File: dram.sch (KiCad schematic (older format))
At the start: 23 parts

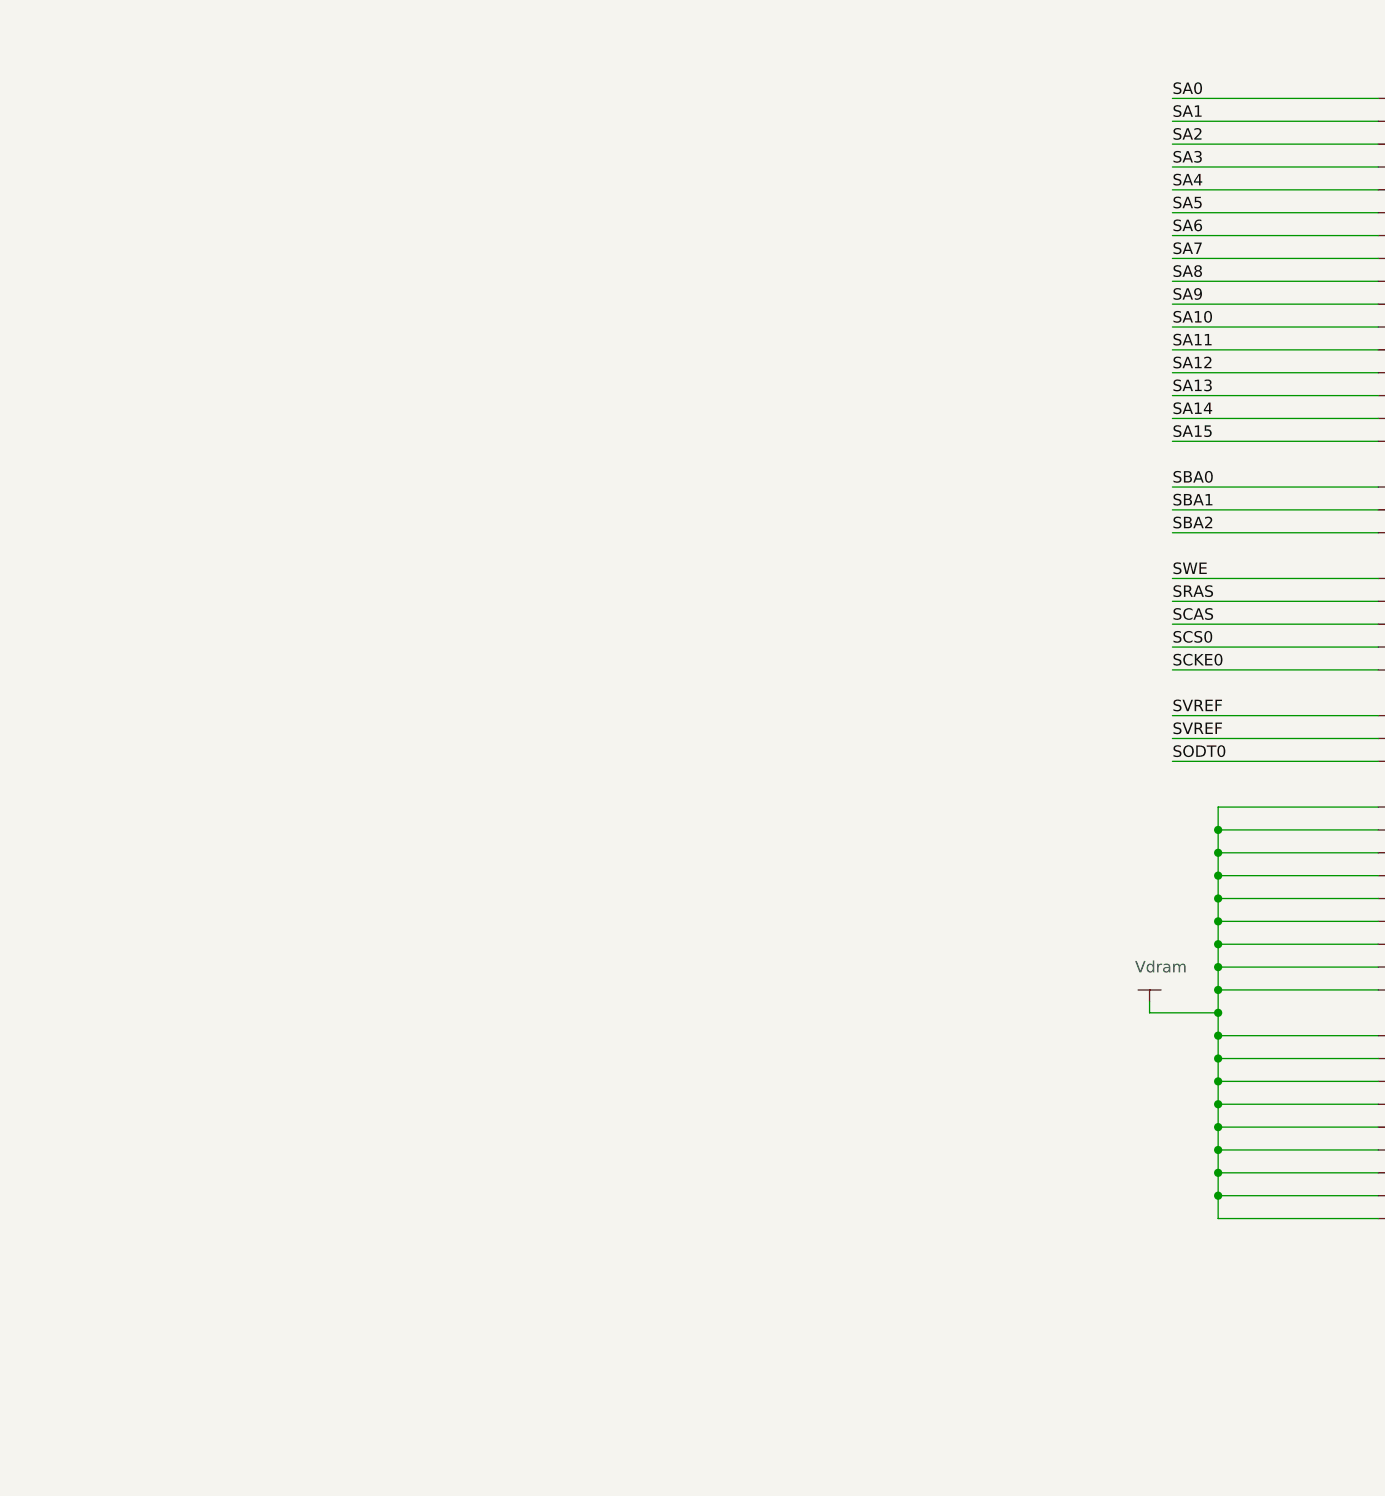
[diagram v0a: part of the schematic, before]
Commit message: update port sys,
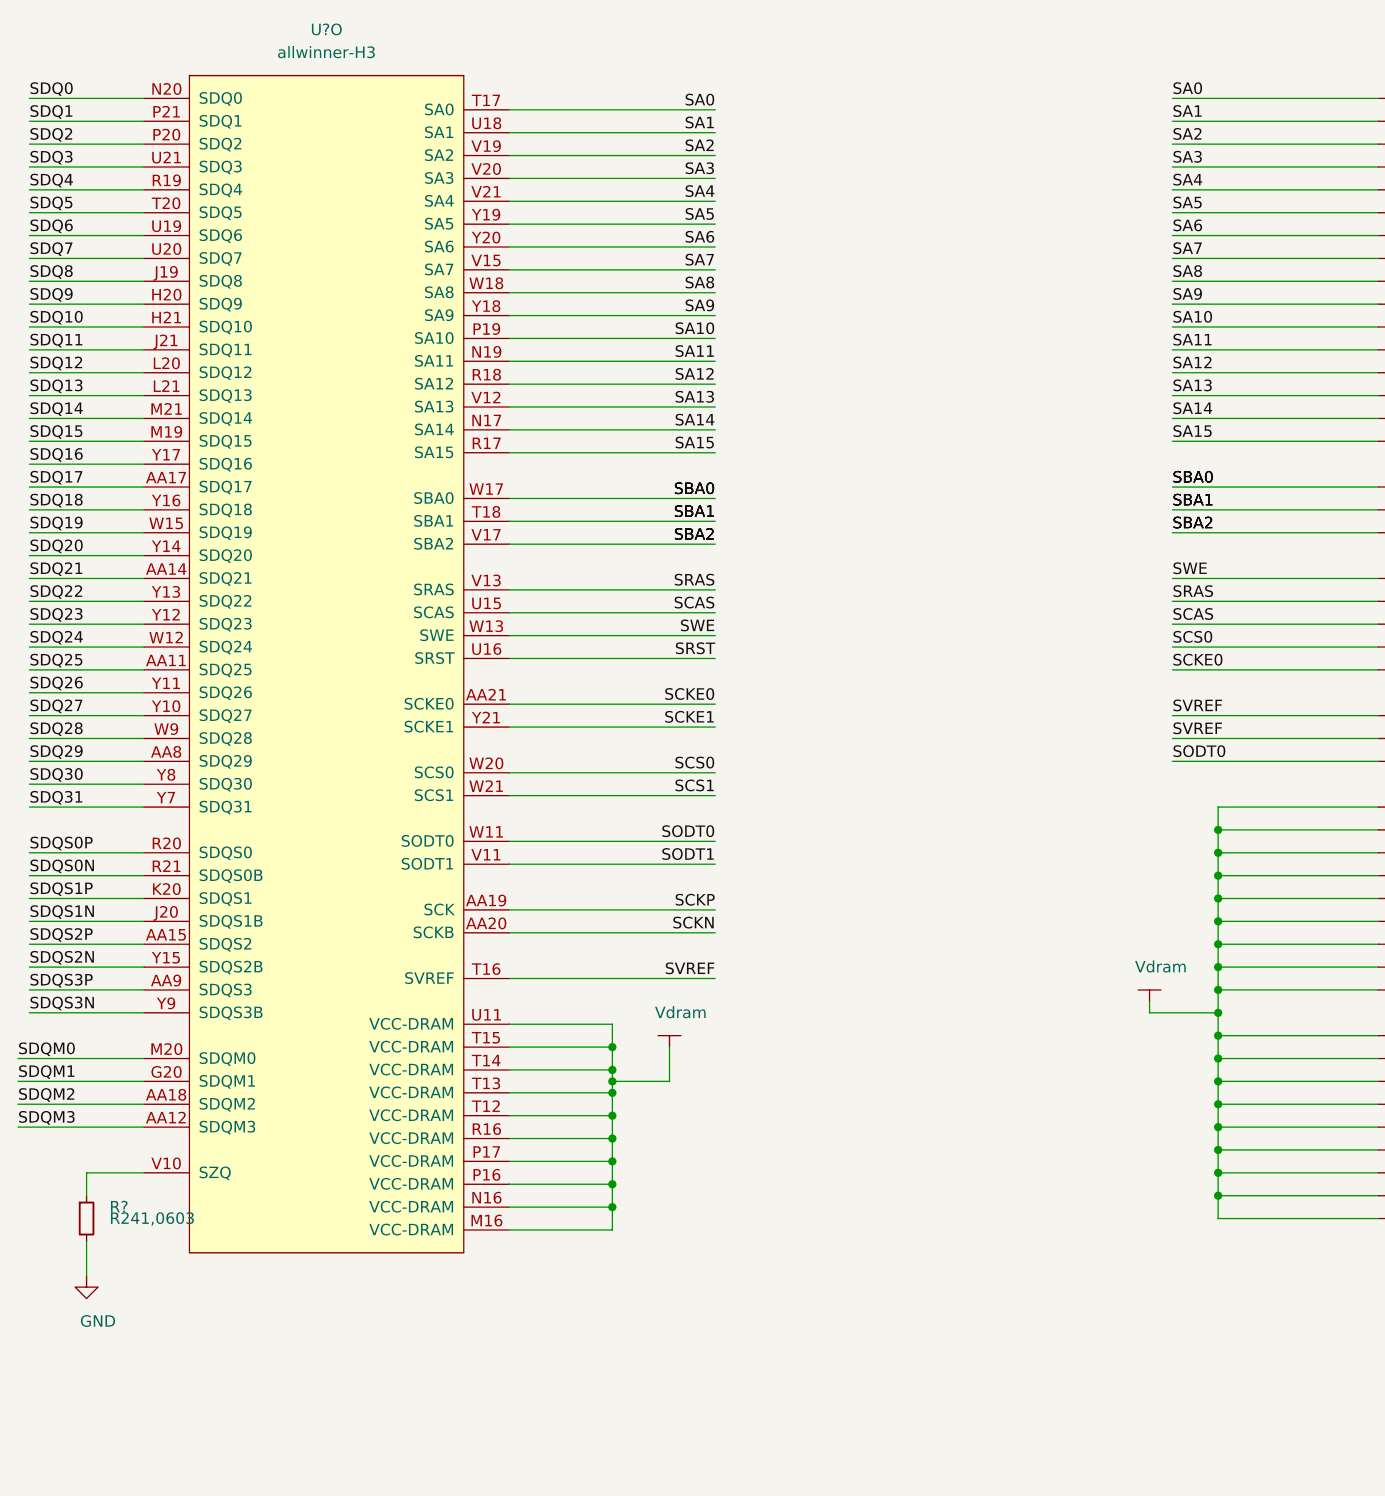
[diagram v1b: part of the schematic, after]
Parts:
- added R?: R241,0603, Resistor_SMD:R_0603_1608Metric_Pad1.05x0.95mm_HandSolder, symbol taobao-r:R241,0603
- added U?: allwinner-H3, symbol taobao-components:allwinner-H3
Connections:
- net GND: now also R?.2
- net SA0: now also U?.T17 (SA0)
- net SA1: now also U?.U18 (SA1)
- net SA10: now also U?.P19 (SA10)
- net SA11: now also U?.N19 (SA11)
- net SA12: now also U?.R18 (SA12)
- net SA13: now also U?.V12 (SA13)
- net SA14: now also U?.N17 (SA14)
- net SA15: now also U?.R17 (SA15)
- net SA2: now also U?.V19 (SA2)
- net SA3: now also U?.V20 (SA3)
- net SA4: now also U?.V21 (SA4)
- net SA5: now also U?.Y19 (SA5)
- net SA6: now also U?.Y20 (SA6)
- net SA7: now also U?.V15 (SA7)
- net SA8: now also U?.W18 (SA8)
- net SA9: now also U?.Y18 (SA9)
- net SBA0: now also U?.W17 (SBA0)
- net SBA1: now also U?.T18 (SBA1)
- net SBA2: now also U?.V17 (SBA2)
- net SCAS: now also U?.U15 (SCAS)
- net SCKE0: now also U?.AA21 (SCKE0)
- net SCKE1: now also U?.Y21 (SCKE1)
- net SCKN: now also U?.AA20 (SCKB)
- net SCKP: now also U?.AA19 (SCK)
- net SCS0: now also U?.W20 (SCS0)
- net SCS1: now also U?.W21 (SCS1)
- net SDQ0: now also U?.N20 (SDQ0)
- net SDQ1: now also U?.P21 (SDQ1)
- net SDQ10: now also U?.H21 (SDQ10)
- net SDQ11: now also U?.J21 (SDQ11)
- net SDQ12: now also U?.L20 (SDQ12)
- net SDQ13: now also U?.L21 (SDQ13)
- net SDQ14: now also U?.M21 (SDQ14)
- net SDQ15: now also U?.M19 (SDQ15)
- net SDQ16: now also U?.Y17 (SDQ16)
- net SDQ17: now also U?.AA17 (SDQ17)
- net SDQ18: now also U?.Y16 (SDQ18)
- net SDQ19: now also U?.W15 (SDQ19)
- net SDQ2: now also U?.P20 (SDQ2)
- net SDQ20: now also U?.Y14 (SDQ20)
- net SDQ21: now also U?.AA14 (SDQ21)
- net SDQ22: now also U?.Y13 (SDQ22)
- net SDQ23: now also U?.Y12 (SDQ23)
- net SDQ24: now also U?.W12 (SDQ24)
- net SDQ25: now also U?.AA11 (SDQ25)
- net SDQ26: now also U?.Y11 (SDQ26)
- net SDQ27: now also U?.Y10 (SDQ27)
- net SDQ28: now also U?.W9 (SDQ28)
- net SDQ29: now also U?.AA8 (SDQ29)
- net SDQ3: now also U?.U21 (SDQ3)
- net SDQ30: now also U?.Y8 (SDQ30)
- net SDQ31: now also U?.Y7 (SDQ31)
- net SDQ4: now also U?.R19 (SDQ4)
- net SDQ5: now also U?.T20 (SDQ5)
- net SDQ6: now also U?.U19 (SDQ6)
- net SDQ7: now also U?.U20 (SDQ7)
- net SDQ8: now also U?.J19 (SDQ8)
- net SDQ9: now also U?.H20 (SDQ9)
- net SDQM0: now also U?.M20 (SDQM0)
- net SDQM1: now also U?.G20 (SDQM1)
- net SDQM2: now also U?.AA18 (SDQM2)
- net SDQM3: now also U?.AA12 (SDQM3)
- net SDQS0N: now also U?.R21 (SDQS0B)
- net SDQS0P: now also U?.R20 (SDQS0)
- net SDQS1N: now also U?.J20 (SDQS1B)
- net SDQS1P: now also U?.K20 (SDQS1)
- net SDQS2N: now also U?.Y15 (SDQS2B)
- net SDQS2P: now also U?.AA15 (SDQS2)
- net SDQS3N: now also U?.Y9 (SDQS3B)
- net SDQS3P: now also U?.AA9 (SDQS3)
- net SODT0: now also U?.W11 (SODT0)
- net SODT1: now also U?.V11 (SODT1)
- net SRAS: now also U?.V13 (SRAS)
- net SRST: now also U?.U16 (SRST)
- net SVREF: now also U?.T16 (SVREF)
- net SWE: now also U?.W13 (SWE)
- net Vdram: now also U?.M16 (VCC-DRAM), U?.N16 (VCC-DRAM), U?.P16 (VCC-DRAM), U?.P17 (VCC-DRAM), U?.R16 (VCC-DRAM), U?.T12 (VCC-DRAM), U?.T13 (VCC-DRAM), U?.T14 (VCC-DRAM), U?.T15 (VCC-DRAM), U?.U11 (VCC-DRAM)
- new net: R?.1, U?.V10 (SZQ)
